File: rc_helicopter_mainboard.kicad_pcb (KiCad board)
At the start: 2 copper layers, 55 x 55 mm, 4 parts

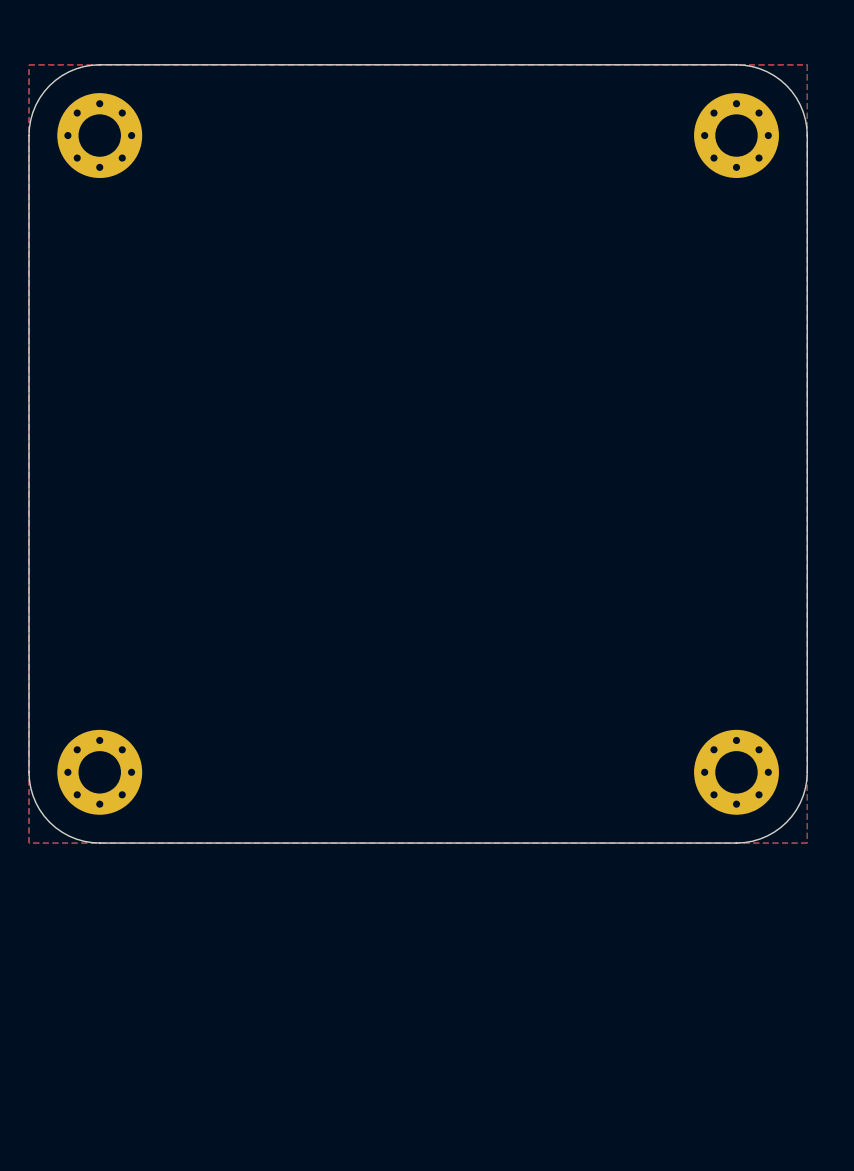
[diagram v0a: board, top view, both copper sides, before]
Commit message: Arrange footprints
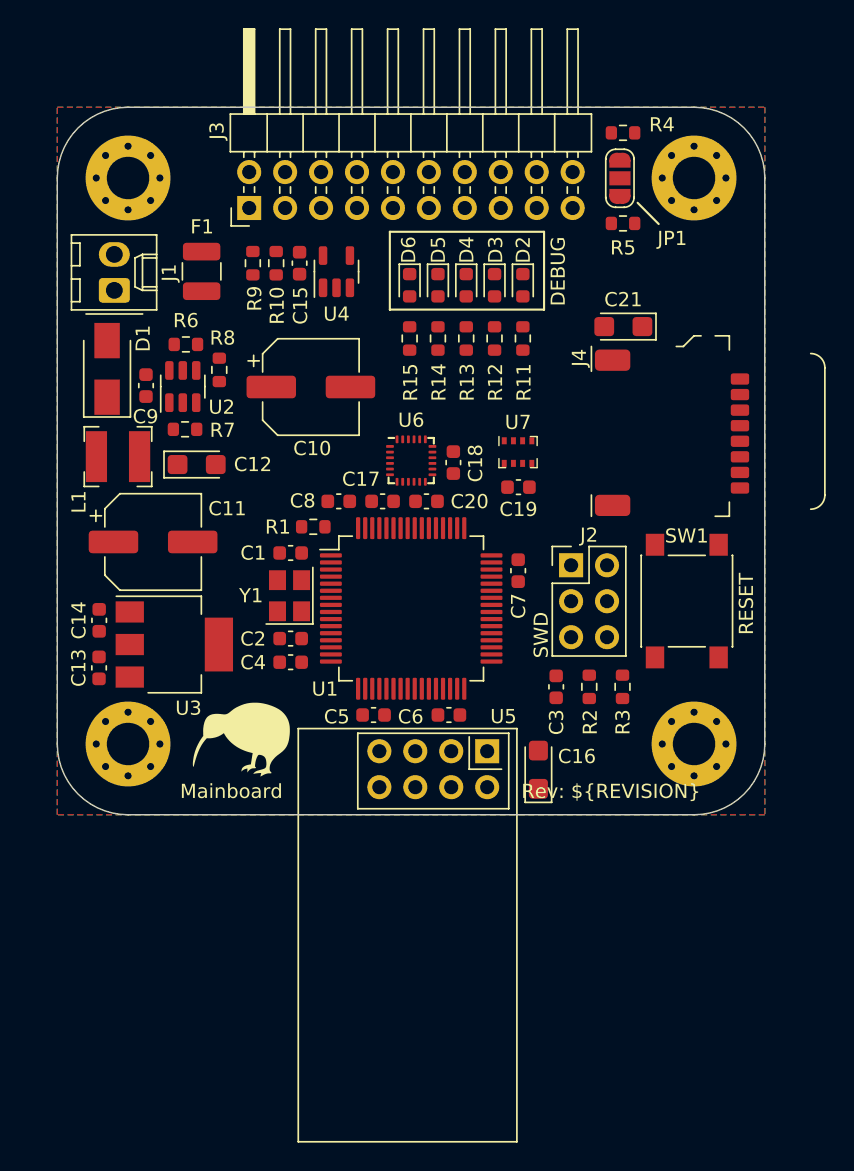
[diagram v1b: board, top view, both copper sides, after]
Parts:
- added C1: 22pF, Capacitor_SMD:C_0603_1608Metric, F.Cu at (138.5, 103.5)
- added C10: 4.7μF, Capacitor_SMD:CP_Elec_6.3x5.4, F.Cu at (139.9, 91.8)
- added C11: 10μF, Capacitor_SMD:CP_Elec_6.3x5.4, F.Cu at (128.8, 102.7)
- added C12: 10μF, Capacitor_Tantalum_SMD:CP_EIA-3216-10_Kemet-I, F.Cu at (131.8, 97.2)
- added C13: 100nF, Capacitor_SMD:C_0603_1608Metric, F.Cu at (125.0, 111.6)
- added C14: 100nF, Capacitor_SMD:C_0603_1608Metric, F.Cu at (125.0, 108.3)
- added C15: 10nF, Capacitor_SMD:C_0603_1608Metric, F.Cu at (139.1, 83.0)
- added C16: 10μF, Capacitor_Tantalum_SMD:CP_EIA-3216-10_Kemet-I, F.Cu at (156.0, 118.8)
- added C17: 100nF, Capacitor_SMD:C_0603_1608Metric, F.Cu at (145.0, 99.8)
- added C18: 100nF, Capacitor_SMD:C_0603_1608Metric, F.Cu at (150.0, 97.1)
- added C19: 100nF, Capacitor_SMD:C_0603_1608Metric, F.Cu at (154.6, 98.8)
- added C2: 22pF, Capacitor_SMD:C_0603_1608Metric, F.Cu at (138.5, 109.5)
- added C20: 100nF, Capacitor_SMD:C_0603_1608Metric, F.Cu at (148.1, 99.8)
- added C21: 4.7μF, Capacitor_Tantalum_SMD:CP_EIA-3216-10_Kemet-I, F.Cu at (162.0, 87.5)
- added C3: 100nF, Capacitor_SMD:C_0603_1608Metric, F.Cu at (157.3, 113.0)
- added C4: 100nF, Capacitor_SMD:C_0603_1608Metric, F.Cu at (138.5, 111.2)
- added C5: 100nF, Capacitor_SMD:C_0603_1608Metric, F.Cu at (144.3, 115.0)
- added C6: 100nF, Capacitor_SMD:C_0603_1608Metric, F.Cu at (149.7, 115.0)
- added C7: 100nF, Capacitor_SMD:C_0603_1608Metric, F.Cu at (154.6, 104.8)
- added C8: 100nF, Capacitor_SMD:C_0603_1608Metric, F.Cu at (141.9, 99.8)
- added C9: 10nF, Capacitor_SMD:C_0603_1608Metric, F.Cu at (128.3, 91.7)
- added D1: SK36A, Diode_SMD:D_SMA, F.Cu at (125.5, 90.5)
- added D2: Blue, LED_SMD:LED_0603_1608Metric, F.Cu at (154.9, 84.6)
- added D3: Blue, LED_SMD:LED_0603_1608Metric, F.Cu at (152.9, 84.6)
- added D4: Blue, LED_SMD:LED_0603_1608Metric, F.Cu at (150.9, 84.6)
- added D5: Blue, LED_SMD:LED_0603_1608Metric, F.Cu at (148.9, 84.6)
- added D6: Blue, LED_SMD:LED_0603_1608Metric, F.Cu at (146.9, 84.6)
- added F1: 1A, Fuse:Fuse_1210_3225Metric, F.Cu at (132.2, 83.6)
- added G***: LOGO, Local_Library:Kiwi, F.Cu at (135.0, 116.7)
- added J1: Battery Pack, Connector_Molex:Molex_KK-254_AE-6410-02A_1x02_P2.54mm_Vertical, F.Cu at (126.0, 84.9)
- added J2: SWD, Connector_PinHeader_2.54mm:PinHeader_2x03_P2.54mm_Vertical, F.Cu at (158.3, 104.4)
- added J3: Main Connector, Connector_PinHeader_2.54mm:PinHeader_2x10_P2.54mm_Horizontal, F.Cu at (135.6, 79.1)
- added J4: Micro_SD_Card, Local_Library:112K-TAA0-RA1, F.Cu at (161.2, 94.4)
- added JP1: SolderJumper_3_Open, Jumper:SolderJumper-3_P1.3mm_Open_RoundedPad1.0x1.5mm_NumberLabels, F.Cu at (161.8, 77.0)
- added L1: 2.2μH, Inductor_SMD:L_Bourns-SRN4018, F.Cu at (126.3, 96.7)
- added R1: 10kΩ, Resistor_SMD:R_0603_1608Metric, F.Cu at (140.1, 101.7)
- added R10: 33kΩ, Resistor_SMD:R_0603_1608Metric, F.Cu at (137.5, 83.0)
- added R11: 140Ω, Resistor_SMD:R_0603_1608Metric, F.Cu at (154.9, 88.3)
- added R12: 140Ω, Resistor_SMD:R_0603_1608Metric, F.Cu at (152.9, 88.3)
- added R13: 140Ω, Resistor_SMD:R_0603_1608Metric, F.Cu at (150.9, 88.3)
- added R14: 140Ω, Resistor_SMD:R_0603_1608Metric, F.Cu at (148.9, 88.3)
- added R15: 140Ω, Resistor_SMD:R_0603_1608Metric, F.Cu at (146.9, 88.3)
- added R2: 10kΩ, Resistor_SMD:R_0603_1608Metric, F.Cu at (159.6, 113.0)
- added R3: 330Ω, Resistor_SMD:R_0603_1608Metric, F.Cu at (161.9, 113.0)
- added R4: 4.7kΩ, Resistor_SMD:R_0603_1608Metric, F.Cu at (162.0, 73.8)
- added R5: 4.7kΩ, Resistor_SMD:R_0603_1608Metric, F.Cu at (162.0, 80.2)
- added R6: 10kΩ, Resistor_SMD:R_0603_1608Metric, F.Cu at (131.1, 88.8)
- added R7: 39kΩ, Resistor_SMD:R_0603_1608Metric, F.Cu at (131.0, 94.8)
- added R8: 7.5kΩ, Resistor_SMD:R_0603_1608Metric, F.Cu at (133.4, 90.6)
- added R9: 100kΩ, Resistor_SMD:R_0603_1608Metric, F.Cu at (135.8, 83.0)
- added SW1: Tactswitch, Button_Switch_SMD:SW_SPST_PTS645, F.Cu at (166.5, 106.9)
- added U1: STM32L4P5RET6, Package_QFP:LQFP-64_10x10mm_P0.5mm, F.Cu at (147.0, 107.4)
- added U2: AOZ1280CI, Package_TO_SOT_SMD:SOT-23-6, F.Cu at (130.9, 91.7)
- added U3: LM1117-3.3, Package_TO_SOT_SMD:SOT-223-3_TabPin2, F.Cu at (130.3, 110.0)
- added U4: LM321, Package_TO_SOT_SMD:SOT-23-5, F.Cu at (141.7, 83.6)
- added U5: NRF24L01_Breakout, RF_Module:nRF24L01_Breakout, F.Cu at (152.4, 117.5)
- added U6: MPU-9250, Sensor_Motion:InvenSense_QFN-24_3x3mm_P0.4mm, F.Cu at (147.0, 97.0)
- added U7: BMP280, Package_LGA:Bosch_LGA-8_2x2.5mm_P0.65mm_ClockwisePinNumbering, F.Cu at (154.6, 96.4)
- added Y1: 16MHz, Crystal:Crystal_SMD_3225-4Pin_3.2x2.5mm, F.Cu at (138.4, 106.5)
- moved REF** 4.24 mm to (167.0, 77.0)
- moved REF** 3.61 mm to (167.0, 117.0)
- moved REF** 3.61 mm to (127.0, 77.0)
- moved REF** 2.83 mm to (127.0, 117.0)
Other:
- board size 55 x 55 mm -> 50 x 50 mm
- board text added: "DEBUG"
- board text added: "Mainboard"
- board text added: "RESET"
- board text added: "Rev: ${REVISION}"
- board text added: "SWD"
